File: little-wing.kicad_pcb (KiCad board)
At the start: 2 copper layers, 119.8 x 94.8 mm, 72 parts, among them IC1 AP7335-WG-7, J1 nice!view, J2 Battery, J3 trackball, J4 trackball, SW1 Power, SW2 Reset, U1 nice!nano v2, U2 PMW3610

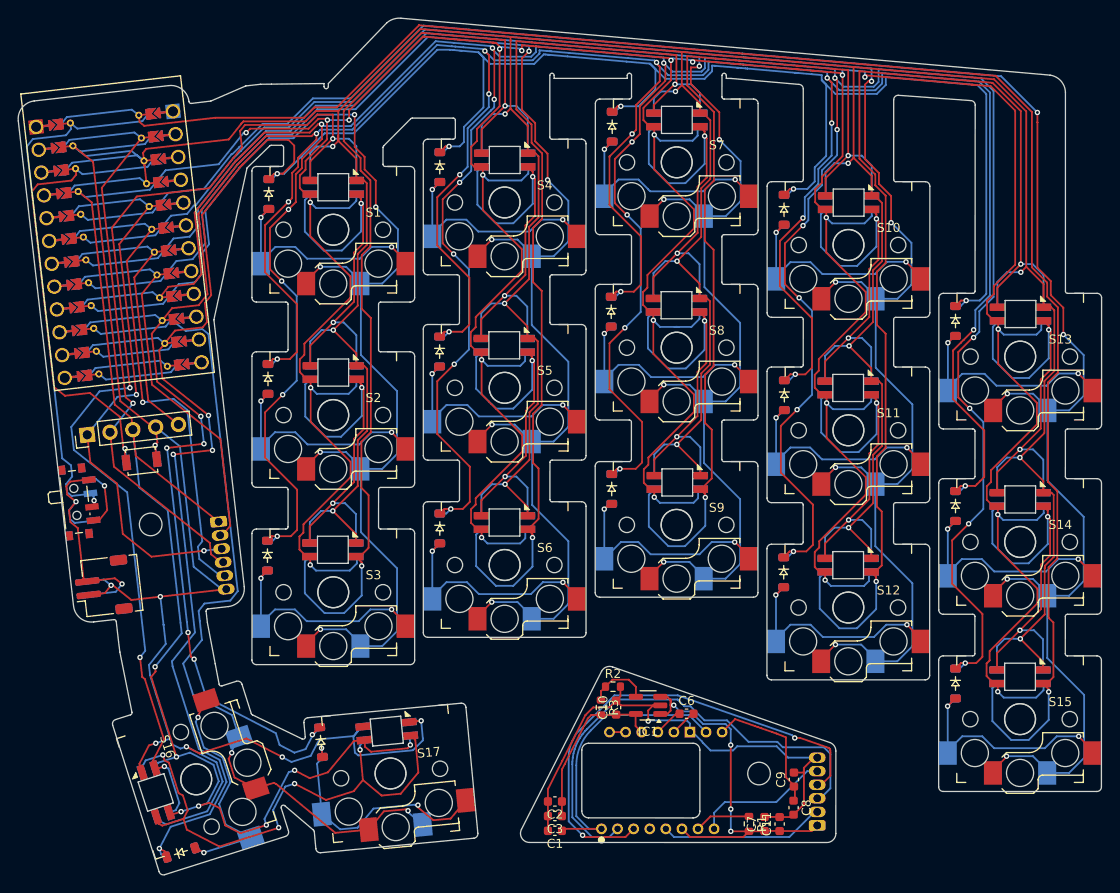
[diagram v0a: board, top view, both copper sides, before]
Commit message: Clearing out all the wiring
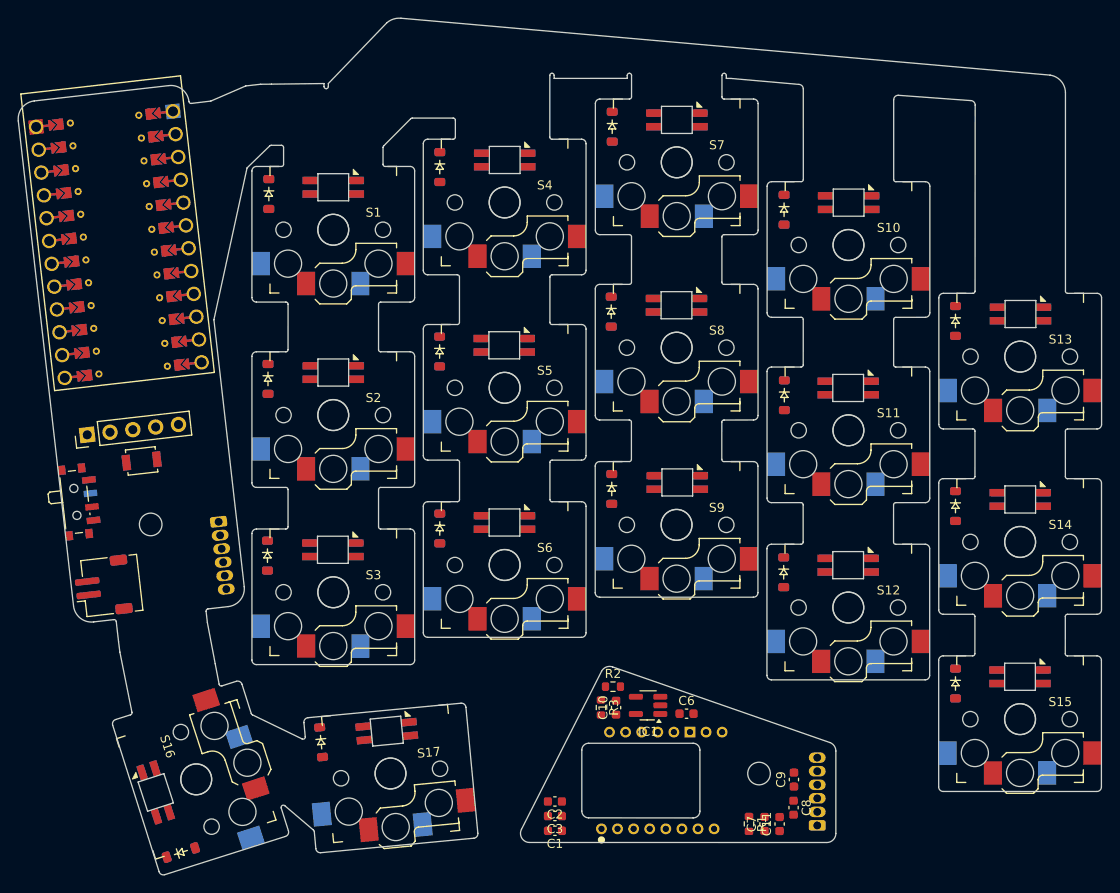
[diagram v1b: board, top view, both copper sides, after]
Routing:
- net GND: track 763.2 -> 0.00 mm, vias 23 -> 0
- net VCC: track 681.9 -> 0.00 mm, vias 31 -> 0
- net Row 0: track 438.6 -> 0.00 mm, vias 26 -> 0
- net Row 1: track 391.8 -> 0.00 mm, vias 22 -> 0
- net Row 2: track 281.6 -> 0.00 mm, vias 9 -> 0
- net Col 0: track 230.3 -> 0.00 mm, vias 5 -> 0
- net Col 1: track 203.0 -> 0.00 mm, vias 5 -> 0
- net RGB: track 199.4 -> 0.00 mm, vias 1 -> 0
- net Col 2: track 178.5 -> 0.00 mm, vias 5 -> 0
- net Col 3: track 166.4 -> 0.00 mm, vias 5 -> 0
- net Col 4: track 142.0 -> 0.00 mm, vias 5 -> 0
- net Net-(D31-DIN): track 124.0 -> 0.00 mm, vias 2 -> 0
- net Net-(D19-DIN): track 121.5 -> 0.00 mm, vias 4 -> 0
- net Net-(D22-DIN): track 111.9 -> 0.00 mm, vias 2 -> 0
- net Net-(D28-DIN): track 107.2 -> 0.00 mm, vias 2 -> 0
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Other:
- copper layers 2 -> 4
